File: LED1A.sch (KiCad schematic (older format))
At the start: 16 parts

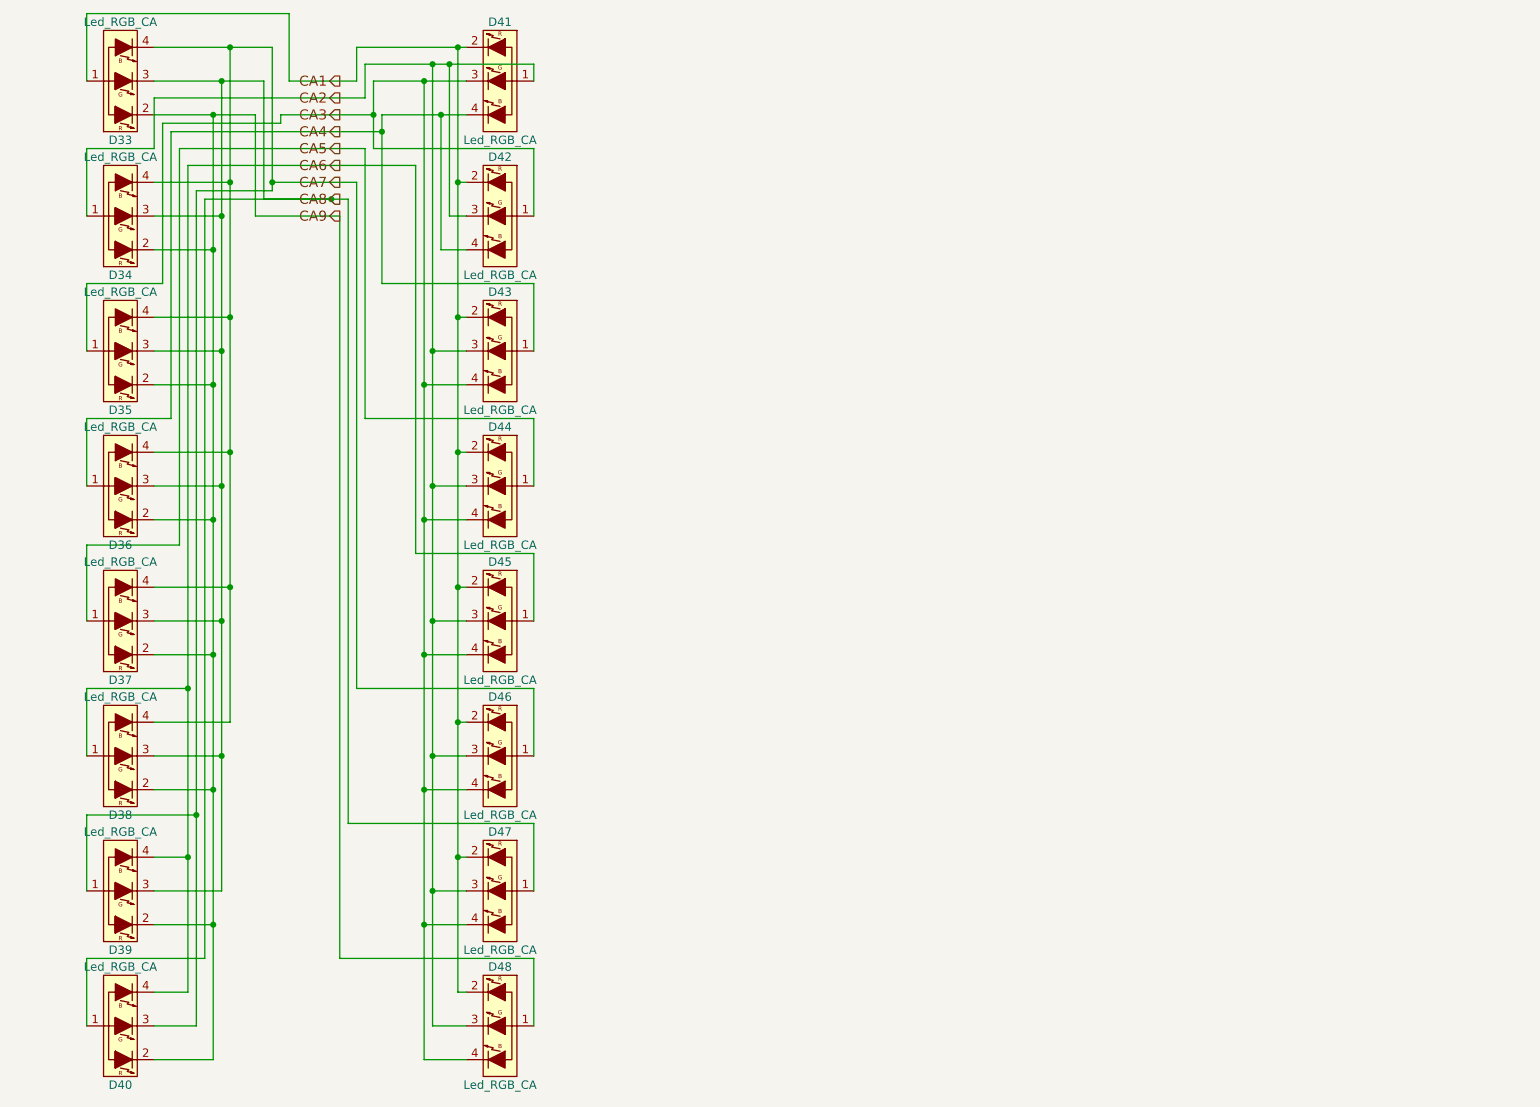
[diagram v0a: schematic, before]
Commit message: Clean up LED-Schematics
Luckily I didn't make any mistakes in the first run.
(Unless I made the same Mistake twice)
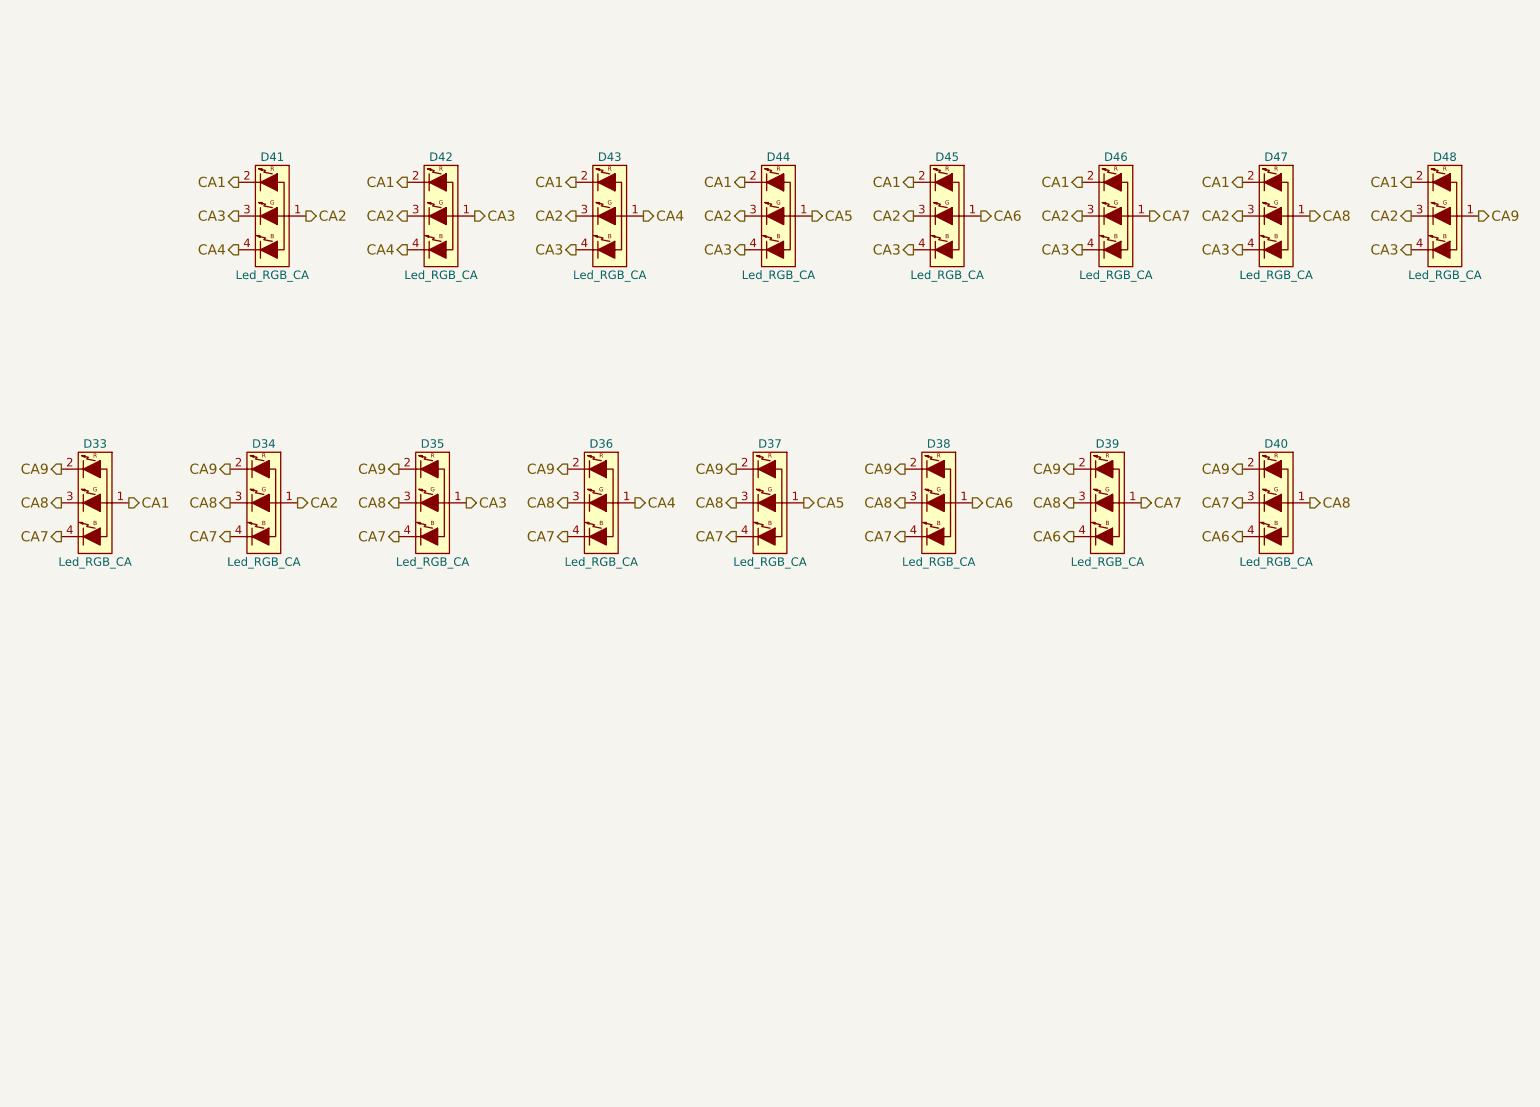
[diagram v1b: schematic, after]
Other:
- moved on the sheet: D33, D34, D35, D36, D37, D38, D39, D40, D41, D42, D43, D44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
